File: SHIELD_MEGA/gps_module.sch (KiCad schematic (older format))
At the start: 1 part

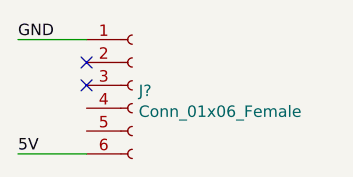
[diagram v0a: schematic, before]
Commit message: GPS pins position defined
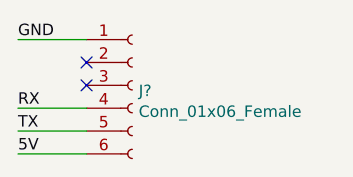
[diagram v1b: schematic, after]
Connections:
- net RX: now reaches J?.4 (Pin_4)
- net TX: now reaches J?.5 (Pin_5)
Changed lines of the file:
@@
 Wire Wire Line
 	5200 3800 5500 3800
+Text Label 5200 3600 0    50   ~ 0
+RX
+Wire Wire Line
+	5200 3600 5500 3600
+Text Label 5200 3700 0    50   ~ 0
+TX
+Wire Wire Line
+	5200 3700 5500 3700
 $EndSCHEMATC
